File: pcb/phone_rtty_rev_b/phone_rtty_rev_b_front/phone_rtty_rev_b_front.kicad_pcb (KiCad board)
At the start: 2 copper layers, 58 x 24 mm, 3 parts

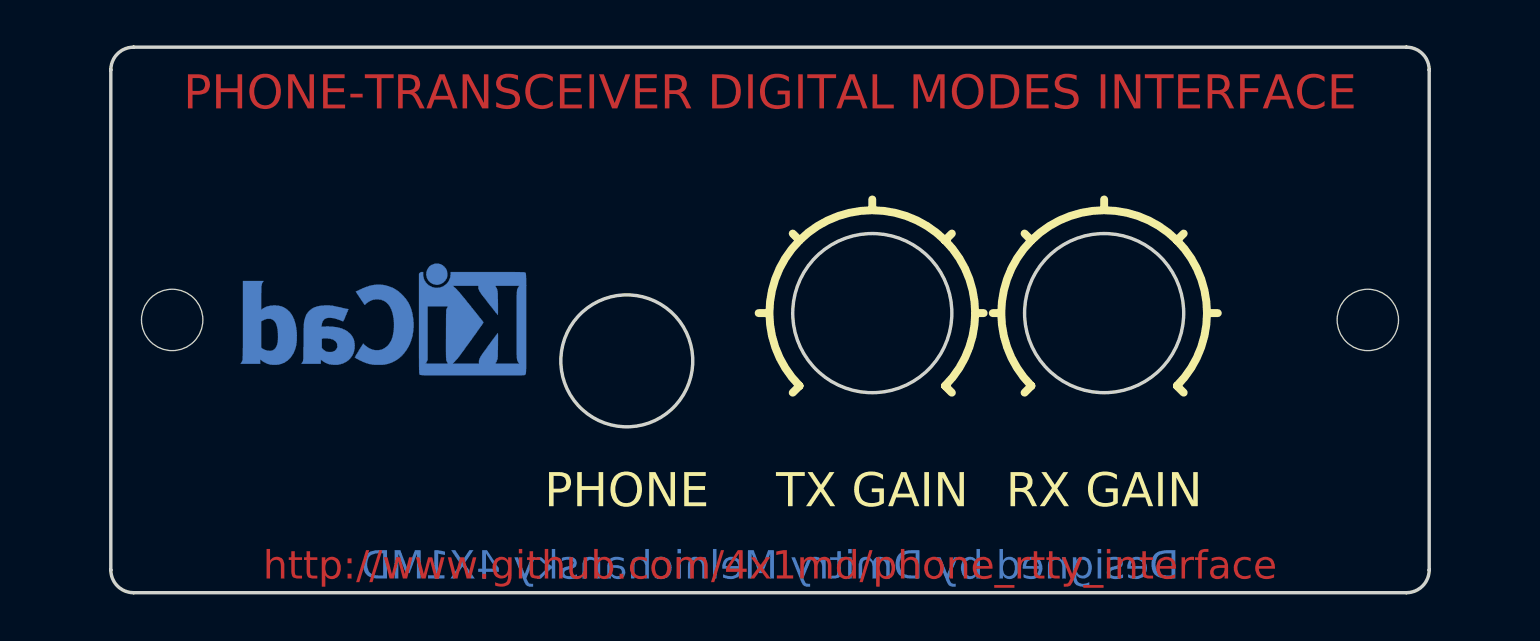
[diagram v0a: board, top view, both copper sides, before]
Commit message: Minor changes.
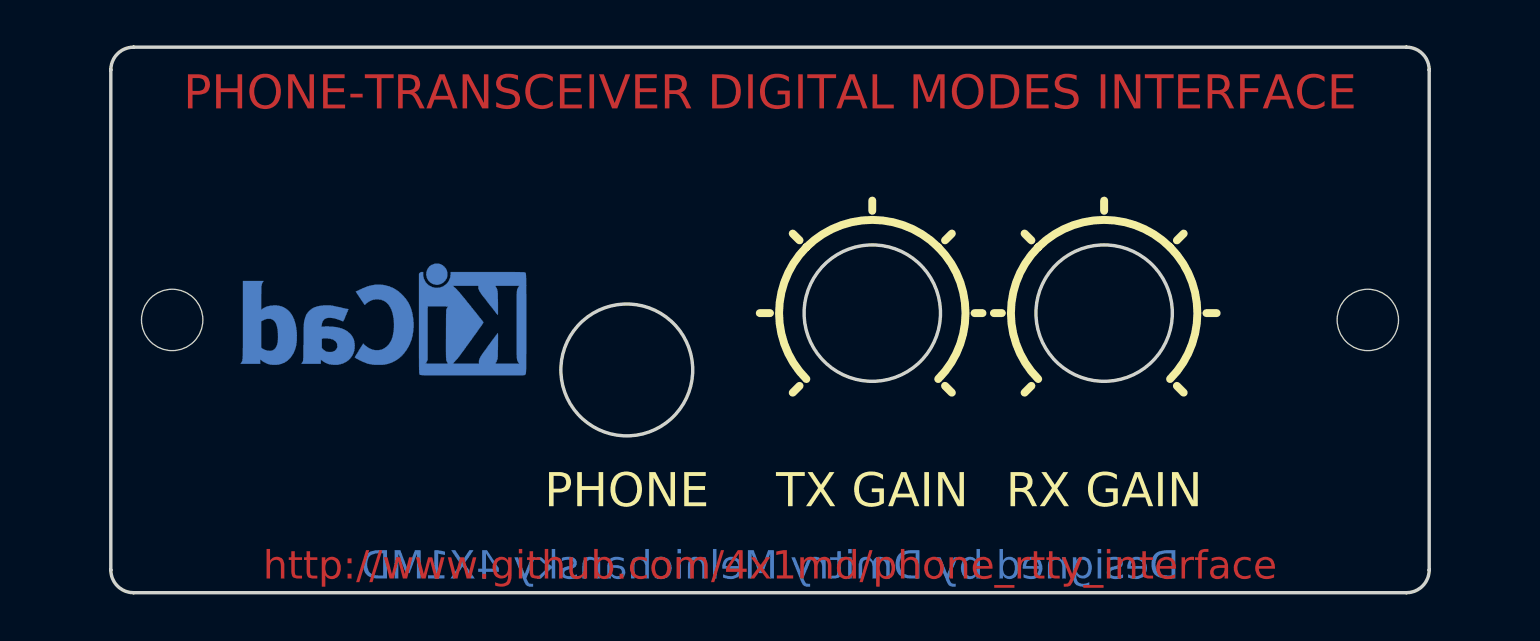
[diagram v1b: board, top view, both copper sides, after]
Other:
- outline, holes or cut-outs redrawn
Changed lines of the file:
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@@
       (xy -2.537313 2.939947) (xy -2.454562 2.96715) (xy -2.376928 2.977424) (xy -2.273043 2.973429)) (layer B.Cu) (width 0.01))
   )
-  (gr_circle (center 133.5 111.7) (end 137 111.7) (layer Edge.Cuts) (width 0.15))
-  (gr_circle (center 143.7 111.7) (end 147.2 111.7) (layer Edge.Cuts) (width 0.15))
-  (gr_line (start 122.7 110.4) (end 122.7 117.2) (angle 90) (layer Dwgs.User) (width 0.05))
+  (gr_arc (start 143.7 111.7) (end 140.8 114.6) (angle 90) (layer F.SilkS) (width 0.35))
+  (gr_arc (start 143.7 111.7) (end 140.8 108.8) (angle 90) (layer F.SilkS) (width 0.35))
+  (gr_arc (start 143.7 111.7) (end 146.6 108.8) (angle 90) (layer F.SilkS) (width 0.35))
+  (gr_arc (start 133.5 111.7) (end 130.6 114.6) (angle 90) (layer F.SilkS) (width 0.35))
+  (gr_arc (start 133.5 111.7) (end 130.6 108.8) (angle 90) (layer F.SilkS) (width 0.35))
+  (gr_arc (start 133.5 111.7) (end 136.4 108.8) (angle 90) (layer F.SilkS) (width 0.35))
+  (gr_circle (center 122.7 114.2) (end 122.7 117.1) (layer Edge.Cuts) (width 0.15))
+  (gr_line (start 122.7 110.8) (end 122.7 117.6) (angle 90) (layer Dwgs.User) (width 0.05))
+  (gr_circle (center 133.5 111.7) (end 136.5 111.7) (layer Edge.Cuts) (width 0.15))
+  (gr_circle (center 143.7 111.7) (end 146.7 111.7) (layer Edge.Cuts) (width 0.15))
   (gr_line (start 140.5 108.5) (end 140.2 108.2) (angle 90) (layer F.SilkS) (width 0.35))
-  (gr_arc (start 143.7 111.7) (end 146.9 108.5) (angle 90) (layer F.SilkS) (width 0.35))
-  (gr_arc (start 143.7 111.7) (end 140.5 108.5) (angle 90) (layer F.SilkS) (width 0.35))
-  (gr_arc (start 143.7 111.7) (end 140.5 114.9) (angle 90) (layer F.SilkS) (width 0.35))
-  (gr_arc (start 133.5 111.7) (end 136.7 108.5) (angle 90) (layer F.SilkS) (width 0.35))
-  (gr_arc (start 133.5 111.7) (end 130.3 108.5) (angle 90) (layer F.SilkS) (width 0.35))
-  (gr_arc (start 133.5 111.7) (end 130.3 114.9) (angle 90) (layer F.SilkS) (width 0.35))
   (gr_line (start 147.2 115.2) (end 140.3 108.3) (angle 90) (layer Dwgs.User) (width 0.05))
   (gr_line (start 140.2 115.2) (end 147.2 108.2) (angle 90) (layer Dwgs.User) (width 0.05))
@@
   (gr_line (start 130 108.2) (end 130.3 108.5) (angle 90) (layer F.SilkS) (width 0.35))
   (gr_line (start 137 108.2) (end 136.7 108.5) (angle 90) (layer F.SilkS) (width 0.35))
-  (gr_line (start 128.5 111.7) (end 128.95 111.7) (angle 90) (layer F.SilkS) (width 0.35))
-  (gr_line (start 133.5 106.7) (end 133.5 107.15) (angle 90) (layer F.SilkS) (width 0.35))
-  (gr_line (start 118.8 113.8) (end 126.6 113.8) (angle 90) (layer Dwgs.User) (width 0.05))
+  (gr_line (start 128.55 111.7) (end 129 111.7) (angle 90) (layer F.SilkS) (width 0.35))
+  (gr_line (start 133.5 106.75) (end 133.5 107.2) (angle 90) (layer F.SilkS) (width 0.35))
+  (gr_line (start 118.8 114.2) (end 126.6 114.2) (angle 90) (layer Dwgs.User) (width 0.05))
   (gr_text "PCB level" (at 152.4 115.9) (layer Cmts.User)
     (effects (font (size 1.2 1.2) (thickness 0.1)))
@@
     (arrow2b (pts (xy 92 111.7) (xy 92.586421 112.826504)))
   )
-  (gr_line (start 138.05 111.7) (end 138.4 111.7) (angle 90) (layer F.SilkS) (width 0.35))
-  (gr_line (start 138.8 111.7) (end 139.15 111.7) (angle 90) (layer F.SilkS) (width 0.35))
-  (gr_line (start 148.25 111.7) (end 148.7 111.7) (angle 90) (layer F.SilkS) (width 0.35))
-  (gr_line (start 143.7 107.15) (end 143.7 106.7) (angle 90) (layer F.SilkS) (width 0.35))
+  (gr_line (start 138 111.7) (end 138.35 111.7) (angle 90) (layer F.SilkS) (width 0.35))
+  (gr_line (start 138.85 111.7) (end 139.2 111.7) (angle 90) (layer F.SilkS) (width 0.35))
+  (gr_line (start 148.2 111.7) (end 148.65 111.7) (angle 90) (layer F.SilkS) (width 0.35))
+  (gr_line (start 143.7 107.2) (end 143.7 106.75) (angle 90) (layer F.SilkS) (width 0.35))
   (gr_text PHONE (at 122.7 119.5) (layer F.SilkS)
     (effects (font (size 1.5 1.5) (thickness 0.3)))
@@
   (gr_line (start 133.5 106.7) (end 133.5 116.7) (angle 90) (layer Dwgs.User) (width 0.05))
   (gr_line (start 127.5 111.7) (end 149.7 111.7) (angle 90) (layer Dwgs.User) (width 0.05))
-  (gr_circle (center 122.7 113.8) (end 125.6 113.7) (layer Edge.Cuts) (width 0.15))
   (dimension 10.2 (width 0.1) (layer Dwgs.User)
     (gr_text "10.200 mm" (at 94.65 118.9 270) (layer Dwgs.User)
